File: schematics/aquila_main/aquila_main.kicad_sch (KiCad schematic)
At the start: 175 parts, among them IC1 MS5611-01BA03, J1 120591-1, J10 PYRO_3, J11 PYRO_2, J12 PYRO_4, J13 PYRO_SAFE, J14 SERVO, J2 1042, J3 1042, J4 PWR, J5 TELEM, J6 GPS, J7 BARO, J8 BMI-S-201, J9 PYRO_1, Q1 IRF7509PbF, Q2 IRF7509PbF, Q3 IRF7509PbF, Q4 IRF7509PbF, U1 LM2576S-3.3/NOPB, U10 MPU-6050, U2 LM2576D2TR4-5G, U3 MAX-M8Q, U4 Si4463, U5 B3520, U6 SKY65723-11, U7 ADXL357, U8 BQ29200, U9 Teensy4.1, Y1 30M

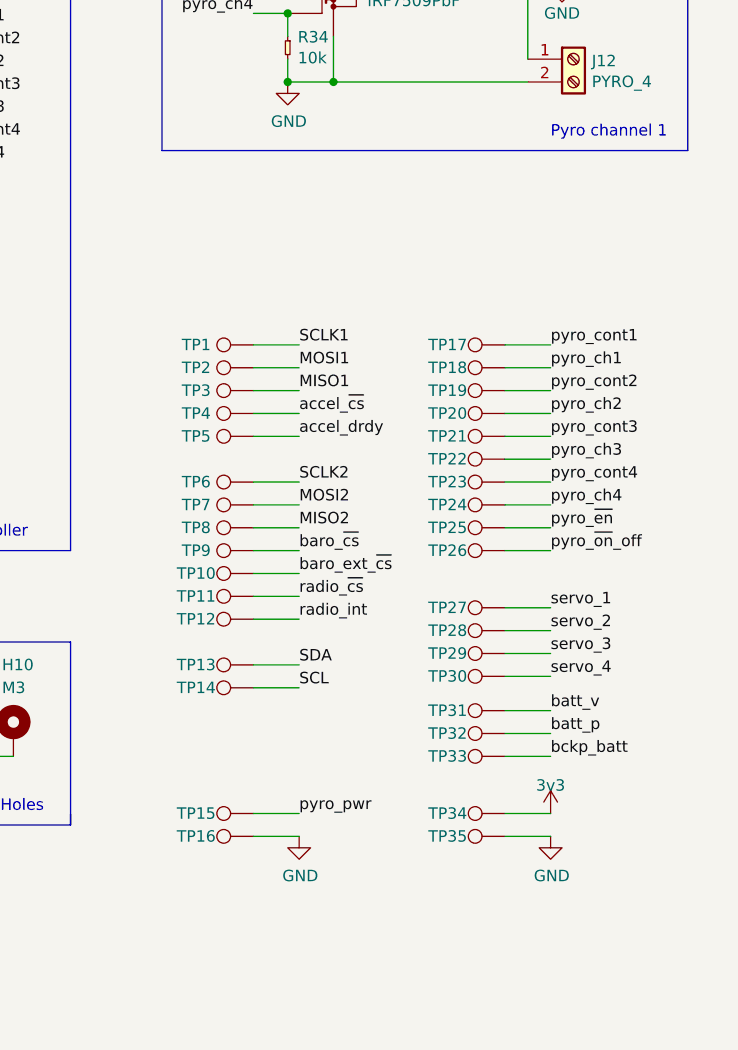
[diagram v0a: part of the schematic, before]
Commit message: added manufacture files and BoM
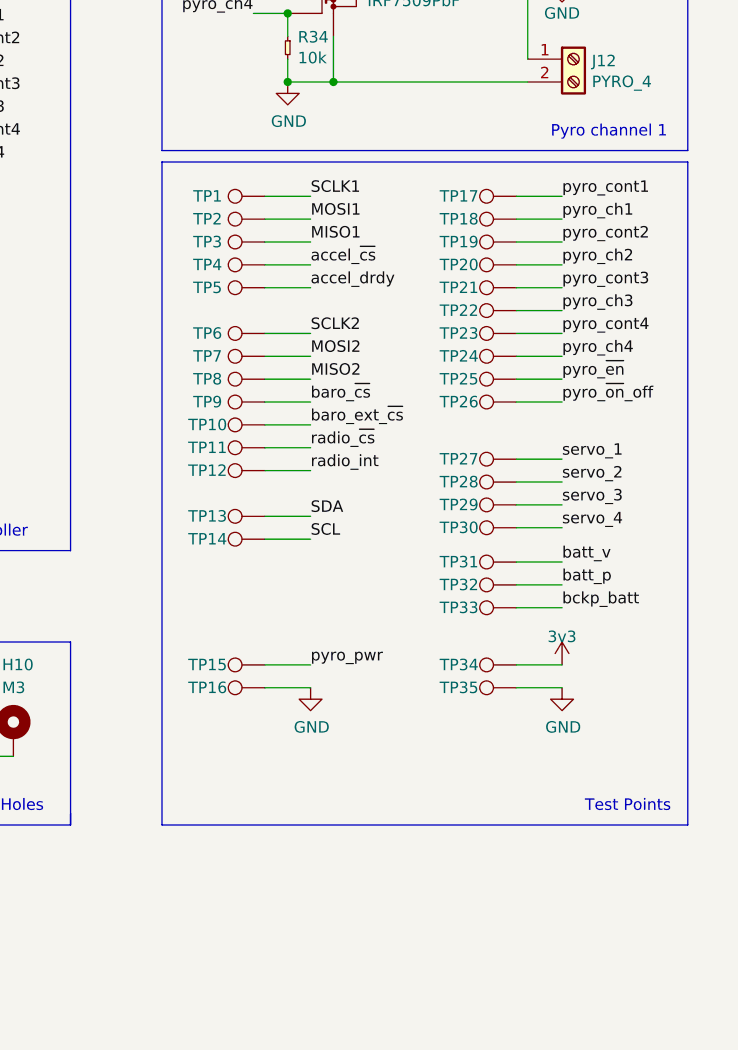
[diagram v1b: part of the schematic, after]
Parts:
- C21, C24: Farnell 3013357 -> 2627406
- J14, J7: DigiKey (none) -> WM16880-ND
- J2, J3: DigiKey 36-1043P-ND -> 36-1042P-ND
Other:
- note added: "Test Points"
- moved on the sheet: TP1, TP10, TP11, TP12, TP13, TP14, TP15, TP16, TP17, TP18, TP19, TP2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
